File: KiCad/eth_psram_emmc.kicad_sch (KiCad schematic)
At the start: 39 parts, among them IC5 MX52LM04A11XVW, IC6 LAN8742A-CZ-TR, IC7 APS256XXN-OBR-BG, Y2 VXM7-9032-25M0000000

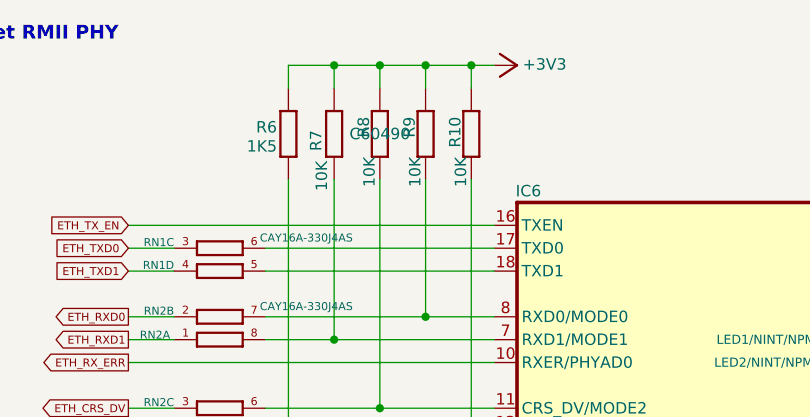
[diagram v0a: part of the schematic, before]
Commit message: BOM update
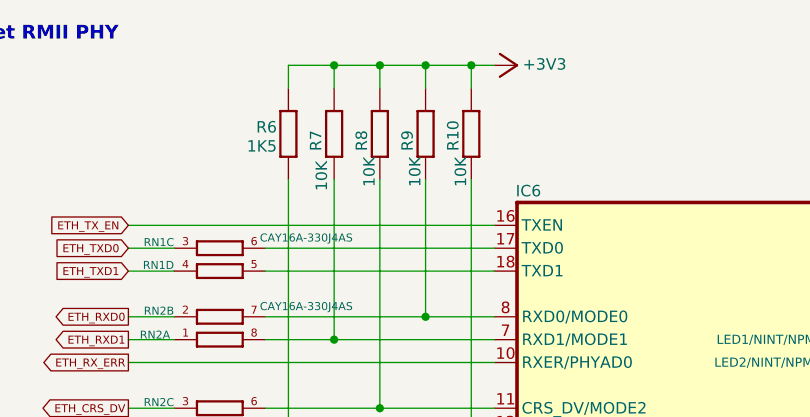
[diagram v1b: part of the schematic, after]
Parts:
- C54, C55, C58, C60: Mouser 187-CL10A475KP8NNNC -> 187-CL10A475KP8NNND
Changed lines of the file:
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@@
 			)
 		)
-		(property "Mouser" "187-CL10A475KP8NNNC"
+		(property "Mouser" "187-CL10A475KP8NNND"
 			(at 256.54 147.32 0)
 			(effects
@@
 			)
 		)
-		(property "Mouser" "187-CL10A475KP8NNNC"
+		(property "Mouser" "187-CL10A475KP8NNND"
 			(at 154.94 73.66 0)
 			(effects
@@
 		(dnp no)
 		(property "Reference" "R8"
-			(at 66.04 26.035 90)
+			(at 67.31 29.845 90)
 			(effects
 				(font
 					(size 1.27 1.27)
 				)
-				(justify right top)
+				(justify left bottom)
 			)
 		)
@@
 					(size 1.27 1.27)
 				)
+				(hide yes)
 			)
 		)
@@
 			)
 		)
-		(property "Mouser" "187-CL10A475KP8NNNC"
+		(property "Mouser" "187-CL10A475KP8NNND"
 			(at 243.84 147.32 0)
 			(effects
@@
 			)
 		)
-		(property "Mouser" "187-CL10A475KP8NNNC"
+		(property "Mouser" "187-CL10A475KP8NNND"
 			(at 167.64 78.74 0)
 			(effects
@@
 		(dnp no)
 		(property "Reference" "R9"
-			(at 71.12 26.035 90)
+			(at 72.39 29.845 90)
 			(effects
 				(font
 					(size 1.27 1.27)
 				)
-				(justify right top)
+				(justify left bottom)
 			)
 		)
@@
 		(dnp no)
 		(property "Reference" "R10"
-			(at 76.2 26.035 90)
+			(at 77.47 29.845 90)
 			(effects
 				(font
 					(size 1.27 1.27)
 				)
-				(justify right top)
+				(justify left bottom)
 			)
 		)
